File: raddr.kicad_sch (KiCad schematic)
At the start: 8 parts, among them J1 Conn_01x03, J2 Conn_01x01, J3 Conn_01x04, J4 Conn_01x01, U1 PMS150C-U06

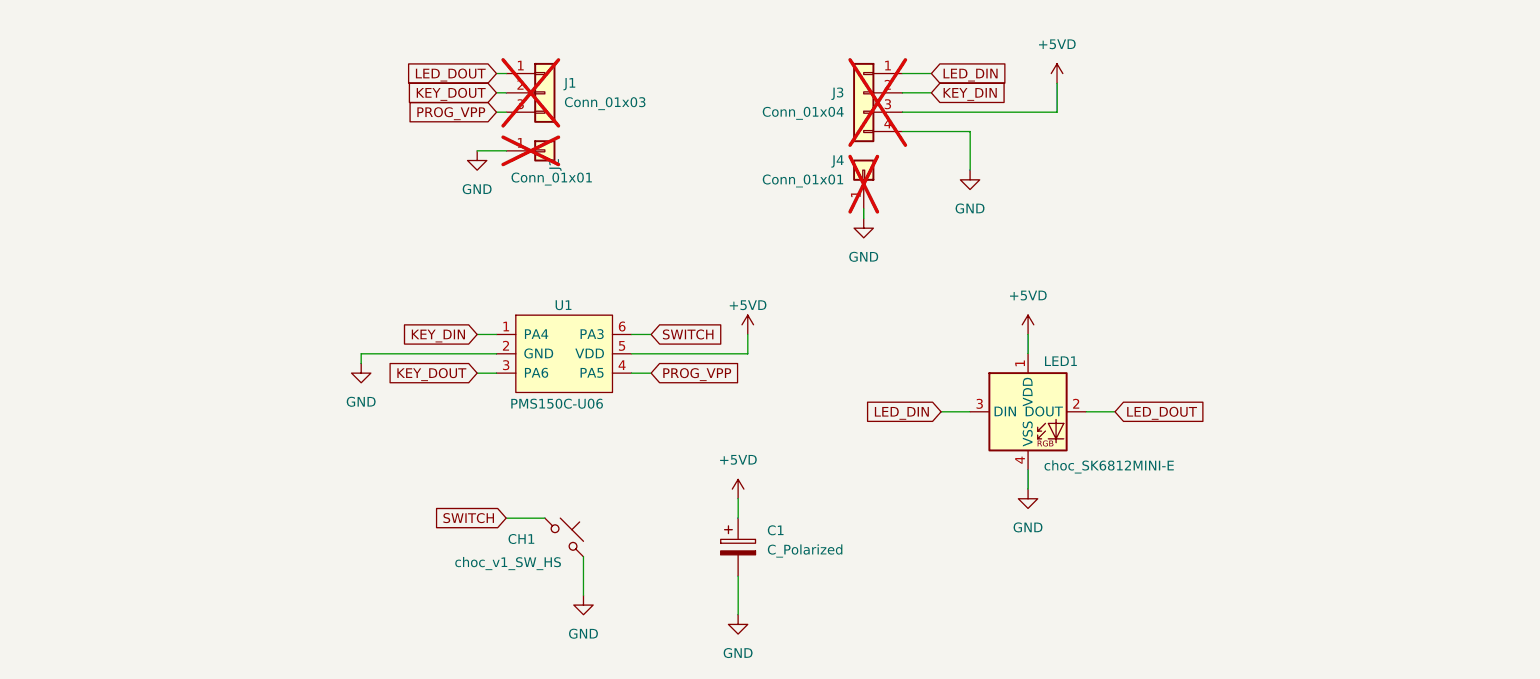
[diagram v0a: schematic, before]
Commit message: Redesign
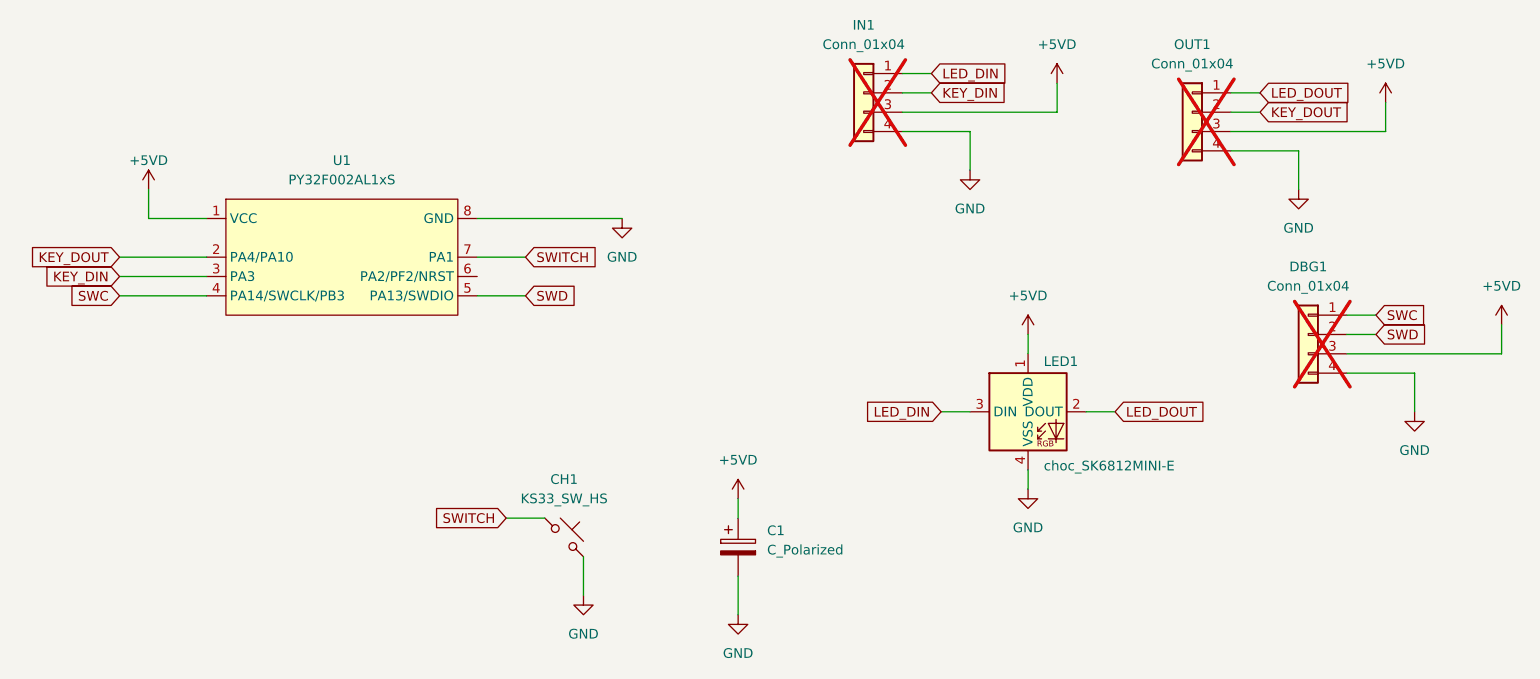
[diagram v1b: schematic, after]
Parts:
- removed CH1: choc_v1_SW_HS, PCM_marbastlib-choc:SW_choc_v1_HS_CPG135001S30_1u, symbol PCM_marbastlib-choc:choc_v1_SW_HS_CPG135001S30
- removed J1: Conn_01x03, Connector_PinSocket_2.54mm:PinSocket_1x03_P2.54mm_Vertical, symbol Connector_Generic:Conn_01x03
- removed J2, J4: Conn_01x01, Connector_PinSocket_2.54mm:PinSocket_1x01_P2.54mm_Vertical, symbol Connector_Generic:Conn_01x01
- removed U1: PMS150C-U06, Package_TO_SOT_SMD:SOT-23-6, symbol Padauk:PMS150C-U06
- added CH1: KS33_SW_HS, PCM_marbastlib-xp-gateron_lp:SW_KS33_HS_KS-2P02B01-02_HS_1u, symbol PCM_marbastlib-gateron_lp:KS33_SW_HS_KS-2P02B01-02
- added DBG1, OUT1: Conn_01x04, Connector_PinSocket_2.54mm:PinSocket_1x04_P2.54mm_Vertical, symbol Connector_Generic:Conn_01x04
- added U1: PY32F002AL1xS, Package_SO:SOP-8_3.9x4.9mm_P1.27mm, symbol MCU_Puya:PY32F002AL1xS
- renumbered J3 to IN1
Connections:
- net +5VD: now also DBG1.3 (Pin_3), OUT1.3 (Pin_3), U1.1 (VCC)
- net GND: now also CH1.2, DBG1.4 (Pin_4), OUT1.4 (Pin_4), U1.8 (GND)
- net KEY_DIN: now also U1.3 (PA3)
- net KEY_DOUT: now also OUT1.2 (Pin_2), U1.2 (PA4/PA10)
- net LED_DOUT: now also OUT1.1 (Pin_1)
- net SWITCH: now also CH1.1, U1.7 (PA1)
- new net SWC: DBG1.1 (Pin_1), U1.4 (PA14/SWCLK/PB3)
- new net SWD: DBG1.2 (Pin_2), U1.5 (PA13/SWDIO)
